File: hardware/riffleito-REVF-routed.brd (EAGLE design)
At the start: 74.2 x 18 mm, 31 parts, among them IC1 ATMEGA328P, IC2 24AA128SN, IC4 MCP1700-33, X1 16 MHz

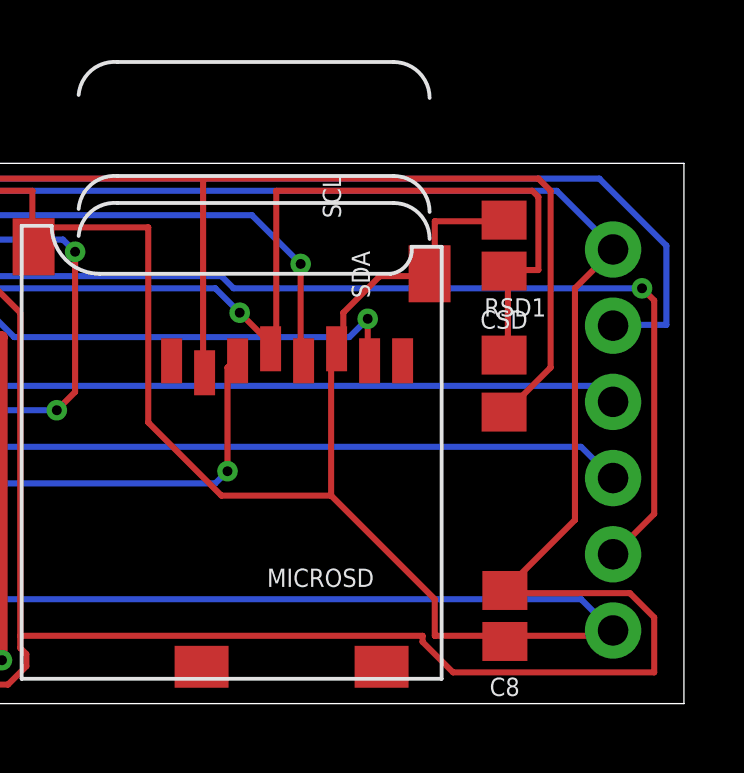
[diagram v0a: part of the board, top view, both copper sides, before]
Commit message: update
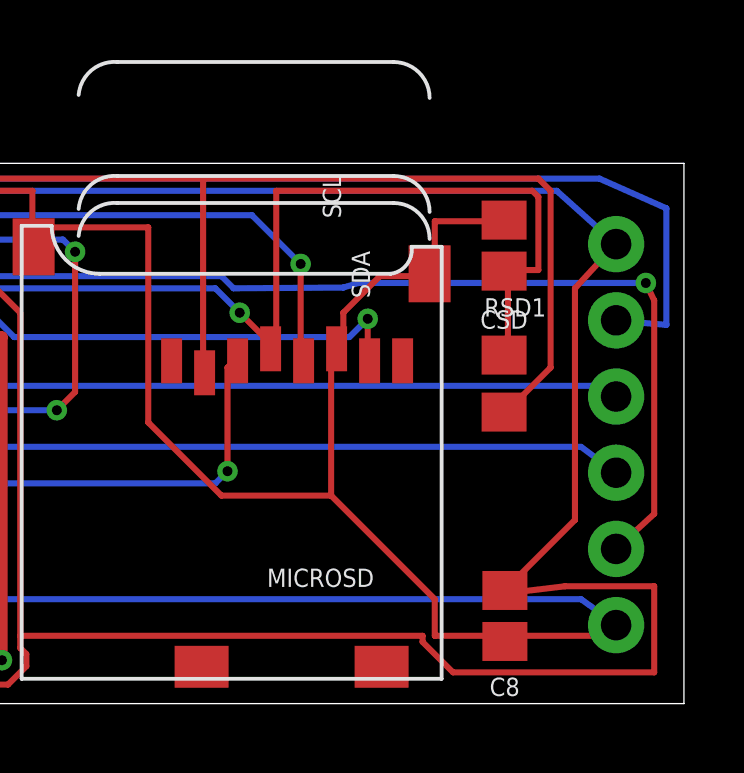
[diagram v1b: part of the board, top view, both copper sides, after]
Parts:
- moved SENSE 0.20 mm to (72.5, 2.59)
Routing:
- net VCC: track 216.0 -> 216.9 mm
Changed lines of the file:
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@@
 <attribute name="VALUE" x="42.5958" y="13.6398" size="1.27" layer="27"/>
 </element>
-<element name="SENSE" library="SparkFun-Connectors" package="1X06" value="" x="72.39" y="2.413" smashed="yes" rot="R90">
-<attribute name="VALUE" x="75.565" y="1.143" size="1.27" layer="27" rot="R90"/>
+<element name="SENSE" library="SparkFun-Connectors" package="1X06" value="" x="72.4916" y="2.5908" smashed="yes" rot="R90">
+<attribute name="VALUE" x="75.6666" y="1.3208" size="1.27" layer="27" rot="R90"/>
 </element>
 <element name="FTDI" library="SparkFun-Connectors" package="1X06" value="" x="2.1336" y="15.3162" smashed="yes" rot="R270">
@@
 <contactref element="JP2" pad="6"/>
 <contactref element="JP1" pad="10"/>
-<wire x1="72.3392" y1="2.2352" x2="68.8848" y2="2.2352" width="0.2032" layer="1"/>
+<wire x1="71.882" y1="2.2352" x2="68.8848" y2="2.2352" width="0.2032" layer="1"/>
 <wire x1="68.8848" y1="2.2352" x2="68.7832" y2="2.0456" width="0.2032" layer="1"/>
-<wire x1="72.3392" y1="2.2352" x2="72.39" y2="2.413" width="0.2032" layer="1"/>
+<wire x1="71.882" y1="2.2352" x2="72.4916" y2="2.5908" width="0.2032" layer="1"/>
 <wire x1="48.5648" y1="16.4592" x2="47.9552" y2="15.8496" width="0.2032" layer="1"/>
 <wire x1="48.5648" y1="16.6624" x2="48.5648" y2="16.4592" width="0.2032" layer="1"/>
@@
 <wire x1="47.3456" y1="2.032" x2="46.5328" y2="1.2192" width="0.2032" layer="16"/>
 <wire x1="47.3456" y1="2.032" x2="47.498" y2="2.2098" width="0.2032" layer="16"/>
-<wire x1="71.3232" y1="3.4544" x2="72.3392" y2="2.4384" width="0.2032" layer="16"/>
+<wire x1="71.3232" y1="3.4544" x2="72.4916" y2="2.6162" width="0.2032" layer="16"/>
 <wire x1="48.768" y1="3.4544" x2="71.3232" y2="3.4544" width="0.2032" layer="16"/>
 <wire x1="47.5488" y1="2.2352" x2="48.768" y2="3.4544" width="0.2032" layer="16"/>
-<wire x1="72.3392" y1="2.4384" x2="72.39" y2="2.413" width="0.2032" layer="16"/>
+<wire x1="72.4916" y1="2.6162" x2="72.4916" y2="2.5908" width="0.2032" layer="16"/>
 <wire x1="47.5488" y1="2.2352" x2="47.498" y2="2.2098" width="0.2032" layer="16"/>
 <via x="19.1008" y="1.4224" extent="1-16" drill="0.3302"/>
@@
 <wire x1="51.4096" y1="10.5664" x2="51.2064" y2="10.7696" width="0.2032" layer="16"/>
 <wire x1="71.9328" y1="10.5664" x2="51.4096" y2="10.5664" width="0.2032" layer="16"/>
-<wire x1="72.3392" y1="10.16" x2="71.9328" y2="10.5664" width="0.2032" layer="16"/>
+<wire x1="72.3392" y1="10.3378" x2="71.9328" y2="10.5664" width="0.2032" layer="16"/>
 <wire x1="20.9296" y1="10.16" x2="20.9296" y2="10.2042" width="0.2032" layer="1"/>
-<wire x1="72.3392" y1="10.16" x2="72.39" y2="10.033" width="0.2032" layer="16"/>
+<wire x1="72.3392" y1="10.3378" x2="72.4916" y2="10.2108" width="0.2032" layer="16"/>
 <via x="19.7104" y="5.2832" extent="1-16" drill="0.3302"/>
 <via x="45.9232" y="4.064" extent="1-16" drill="0.3302"/>
@@
 <wire x1="71.12" y1="6.096" x2="68.8848" y2="3.8608" width="0.2032" layer="1"/>
 <wire x1="71.12" y1="13.8176" x2="71.12" y2="6.096" width="0.2032" layer="1"/>
-<wire x1="72.3392" y1="15.0368" x2="71.12" y2="13.8176" width="0.2032" layer="1"/>
+<wire x1="72.3138" y1="15.113" x2="71.12" y2="13.8176" width="0.2032" layer="1"/>
 <wire x1="68.8848" y1="3.8608" x2="68.7832" y2="3.7456" width="0.2032" layer="1"/>
-<wire x1="72.3392" y1="15.0368" x2="72.39" y2="15.113" width="0.2032" layer="1"/>
+<wire x1="72.3138" y1="15.113" x2="72.4916" y2="15.2908" width="0.2032" layer="1"/>
 <wire x1="36.7792" y1="15.0368" x2="36.576" y2="14.8336" width="0.2032" layer="1"/>
 <wire x1="36.7792" y1="16.4592" x2="36.7792" y2="15.0368" width="0.2032" layer="1"/>
 <wire x1="37.3888" y1="17.0688" x2="36.7792" y2="16.4592" width="0.2032" layer="16"/>
 <wire x1="70.5104" y1="17.0688" x2="37.3888" y2="17.0688" width="0.2032" layer="16"/>
-<wire x1="72.3392" y1="15.24" x2="70.5104" y2="17.0688" width="0.2032" layer="16"/>
-<wire x1="72.3392" y1="15.24" x2="72.39" y2="15.113" width="0.2032" layer="16"/>
+<wire x1="72.263" y1="15.494" x2="70.5104" y2="17.0688" width="0.2032" layer="16"/>
+<wire x1="72.263" y1="15.494" x2="72.4916" y2="15.2908" width="0.2032" layer="16"/>
 <wire x1="66.04" y1="2.2352" x2="52.6288" y2="2.2352" width="0.2032" layer="1"/>
 <wire x1="66.04" y1="2.032" x2="66.04" y2="2.2352" width="0.2032" layer="1"/>
 <wire x1="67.056" y1="1.016" x2="66.04" y2="2.032" width="0.2032" layer="1"/>
 <wire x1="73.7616" y1="1.016" x2="67.056" y2="1.016" width="0.2032" layer="1"/>
-<wire x1="73.7616" y1="2.8448" x2="73.7616" y2="1.016" width="0.2032" layer="1"/>
-<wire x1="72.9488" y1="3.6576" x2="73.7616" y2="2.8448" width="0.2032" layer="1"/>
-<wire x1="68.8848" y1="3.6576" x2="72.9488" y2="3.6576" width="0.2032" layer="1"/>
+<wire x1="73.7616" y1="3.8862" x2="73.7616" y2="1.016" width="0.2032" layer="1"/>
+<wire x1="70.7898" y1="3.8862" x2="73.7616" y2="3.8862" width="0.2032" layer="1"/>
+<wire x1="68.8848" y1="3.6576" x2="70.7898" y2="3.8862" width="0.2032" layer="1"/>
 <wire x1="68.8848" y1="3.6576" x2="68.7832" y2="3.7456" width="0.2032" layer="1"/>
 <wire x1="26.6192" y1="2.8448" x2="24.9936" y2="4.4704" width="0.2032" layer="1"/>
@@
 <wire x1="36.7792" y1="17.4752" x2="35.56" y2="16.256" width="0.2032" layer="16"/>
 <wire x1="71.9328" y1="17.4752" x2="36.7792" y2="17.4752" width="0.2032" layer="16"/>
-<wire x1="74.168" y1="15.24" x2="71.9328" y2="17.4752" width="0.2032" layer="16"/>
-<wire x1="74.168" y1="12.5984" x2="74.168" y2="15.24" width="0.2032" layer="16"/>
-<wire x1="72.5424" y1="12.5984" x2="74.168" y2="12.5984" width="0.2032" layer="16"/>
+<wire x1="74.168" y1="16.4846" x2="71.9328" y2="17.4752" width="0.2032" layer="16"/>
+<wire x1="74.168" y1="12.5984" x2="74.168" y2="16.4846" width="0.2032" layer="16"/>
+<wire x1="72.6694" y1="12.7254" x2="74.168" y2="12.5984" width="0.2032" layer="16"/>
 <wire x1="20.9296" y1="11.176" x2="20.9296" y2="11.0042" width="0.2032" layer="1"/>
-<wire x1="72.5424" y1="12.5984" x2="72.39" y2="12.573" width="0.2032" layer="16"/>
+<wire x1="72.6694" y1="12.7254" x2="72.4916" y2="12.7508" width="0.2032" layer="16"/>
 <via x="22.5552" y="12.8016" extent="1-16" drill="0.3302"/>
 </signal>
@@
 <wire x1="44.2976" y1="16.0528" x2="44.1808" y2="16.1798" width="0.2032" layer="1"/>
 <wire x1="44.2976" y1="10.5664" x2="44.4754" y2="10.5248" width="0.2032" layer="1"/>
-<wire x1="71.3232" y1="8.5344" x2="72.3392" y2="7.5184" width="0.2032" layer="16"/>
+<wire x1="71.3232" y1="8.5344" x2="72.4408" y2="7.6962" width="0.2032" layer="16"/>
 <wire x1="45.9232" y1="8.5344" x2="46.5328" y2="8.5344" width="0.2032" layer="16"/>
 <wire x1="46.5328" y1="8.5344" x2="71.3232" y2="8.5344" width="0.2032" layer="16"/>
 <wire x1="44.5008" y1="9.9568" x2="45.9232" y2="8.5344" width="0.2032" layer="1"/>
 <wire x1="44.5008" y1="10.3632" x2="44.5008" y2="9.9568" width="0.2032" layer="1"/>
-<wire x1="72.3392" y1="7.5184" x2="72.39" y2="7.493" width="0.2032" layer="16"/>
+<wire x1="72.4408" y1="7.6962" x2="72.4916" y2="7.6708" width="0.2032" layer="16"/>
 <wire x1="44.5008" y1="10.3632" x2="44.4754" y2="10.5248" width="0.2032" layer="1"/>
 <wire x1="36.576" y1="7.112" x2="34.7472" y2="5.2832" width="0.2032" layer="1"/>
@@
 <wire x1="36.576" y1="2.6416" x2="36.5506" y2="2.5654" width="0.2032" layer="1"/>
 <wire x1="37.7952" y1="16.0528" x2="37.9882" y2="16.1798" width="0.2032" layer="1"/>
-<wire x1="73.7616" y1="6.2992" x2="72.5424" y2="5.08" width="0.2032" layer="1"/>
+<wire x1="73.7616" y1="6.2992" x2="72.5424" y2="5.1816" width="0.2032" layer="1"/>
 <wire x1="73.7616" y1="13.4112" x2="73.7616" y2="6.2992" width="0.2032" layer="1"/>
-<wire x1="73.3552" y1="13.8176" x2="73.7616" y2="13.4112" width="0.2032" layer="1"/>
-<wire x1="59.7408" y1="13.8176" x2="73.3552" y2="13.8176" width="0.2032" layer="16"/>
+<wire x1="73.4822" y1="13.9954" x2="73.7616" y2="13.4112" width="0.2032" layer="1"/>
+<wire x1="59.7408" y1="13.8176" x2="63.3984" y2="13.843" width="0.2032" layer="16"/>
+<wire x1="63.3984" y1="13.843" x2="63.9064" y2="13.9954" width="0.2032" layer="16"/>
+<wire x1="63.9064" y1="13.9954" x2="73.4822" y2="13.9954" width="0.2032" layer="16"/>
 <wire x1="59.3344" y1="14.224" x2="59.7408" y2="13.8176" width="0.2032" layer="16"/>
 <wire x1="43.0784" y1="14.224" x2="59.3344" y2="14.224" width="0.2032" layer="16"/>
 <wire x1="41.656" y1="12.8016" x2="43.0784" y2="14.224" width="0.2032" layer="1"/>
-<wire x1="72.5424" y1="5.08" x2="72.39" y2="4.953" width="0.2032" layer="1"/>
+<wire x1="72.5424" y1="5.1816" x2="72.4916" y2="5.1308" width="0.2032" layer="1"/>
 <via x="17.0688" y="14.6304" extent="1-16" drill="0.3302"/>
 <via x="31.0896" y="17.0688" extent="1-16" drill="0.3302"/>
-<via x="73.3552" y="13.8176" extent="1-16" drill="0.3302"/>
+<via x="73.4822" y="13.9954" extent="1-16" drill="0.3302"/>
 <via x="43.0784" y="14.224" extent="1-16" drill="0.3302"/>
 </signal>

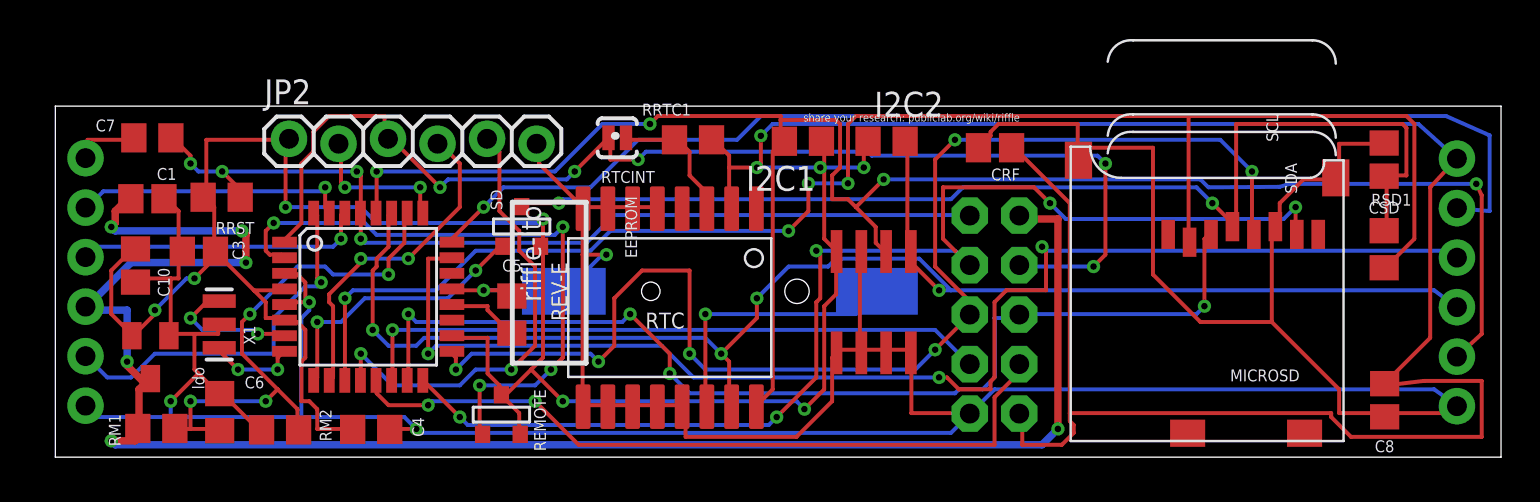
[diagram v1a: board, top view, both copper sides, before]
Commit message: update
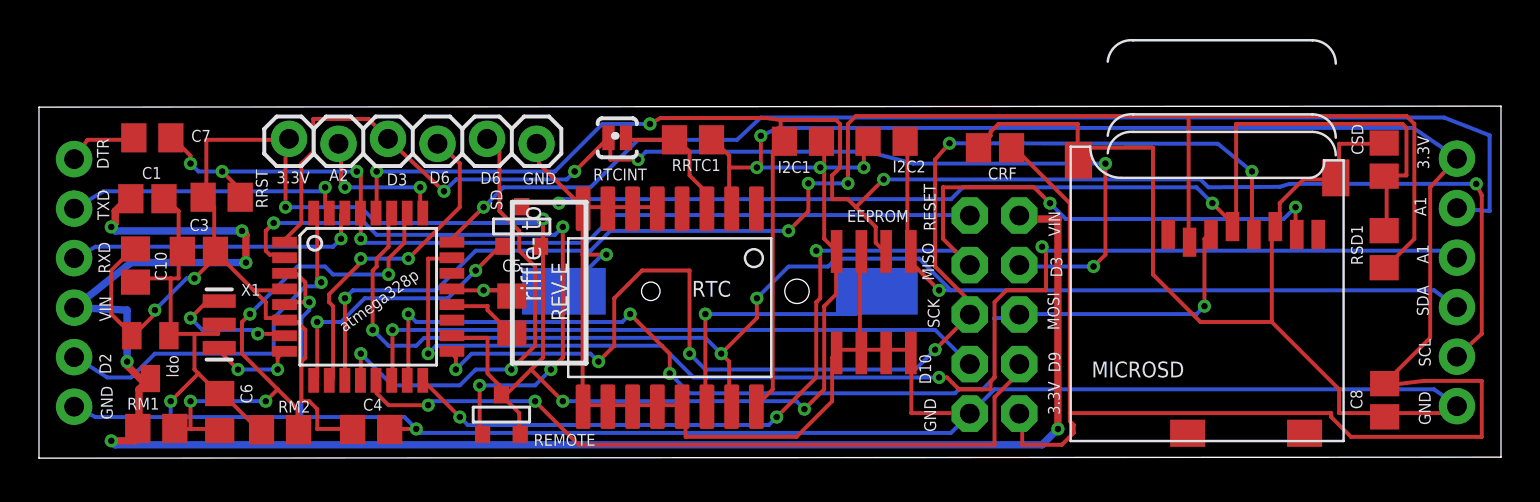
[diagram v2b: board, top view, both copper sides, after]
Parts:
- moved FTDI 0.59 mm to (1.55, 15.3)
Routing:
- net VIN: track 92.9 -> 93.8 mm
- net D3: track 61.4 -> 60.9 mm
- net RXD: track 14.9 -> 15.4 mm
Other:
- board size 74.2 x 18 mm -> 75 x 18.1 mm
- board text added: "A1"
- board text added: "A2"
- board text added: "D10"
- board text added: "D2"
- board text added: "D3"
- board text added: "D9"
- board text added: "DTR"
- board text added: "RXD"
- board text added: "TXD"
- board text added: "atmega328p"
- board text removed: "CERN Open Hardware License Ver. 1.2"
- board text removed: "D8"
- board text removed: "share your research: publiclab.org/wiki/riffle"
